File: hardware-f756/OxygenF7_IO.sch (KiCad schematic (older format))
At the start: 25 parts, among them J10 Micro_SD_Card_Det, J3 JST SH-4, J4 JST ZH-4, J5 Conn_03x08, J6 Conn_01x16, J7 Conn_01x04, J9 1.25mm, U3 MPU-6000, U4 BMP388, U5 W25Q128JVS

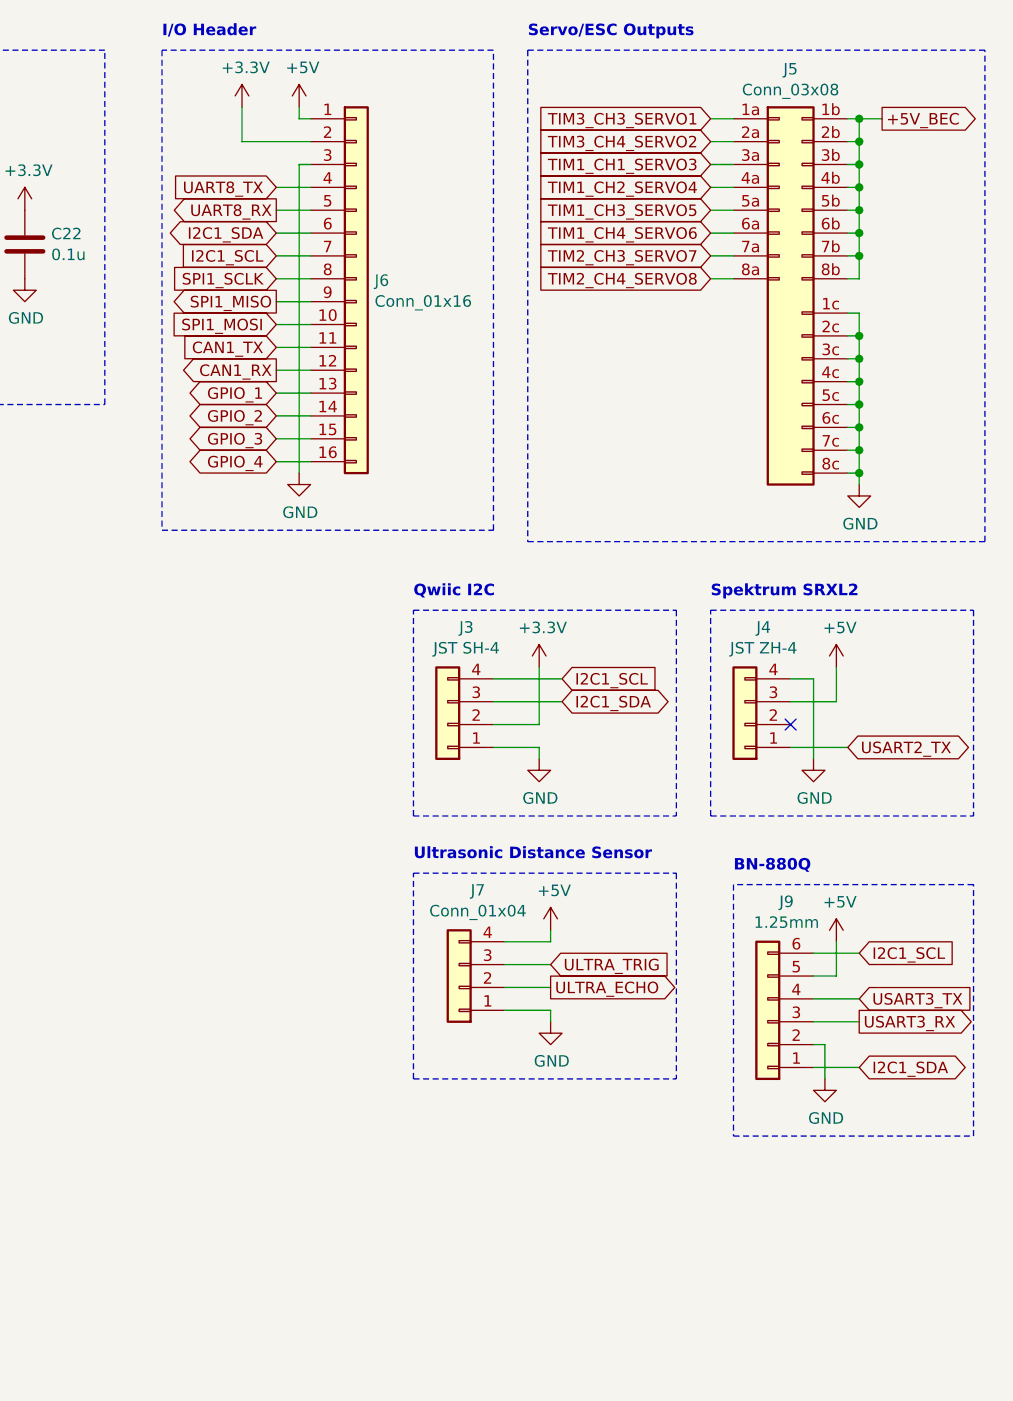
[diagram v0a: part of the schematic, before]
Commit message: New board layout
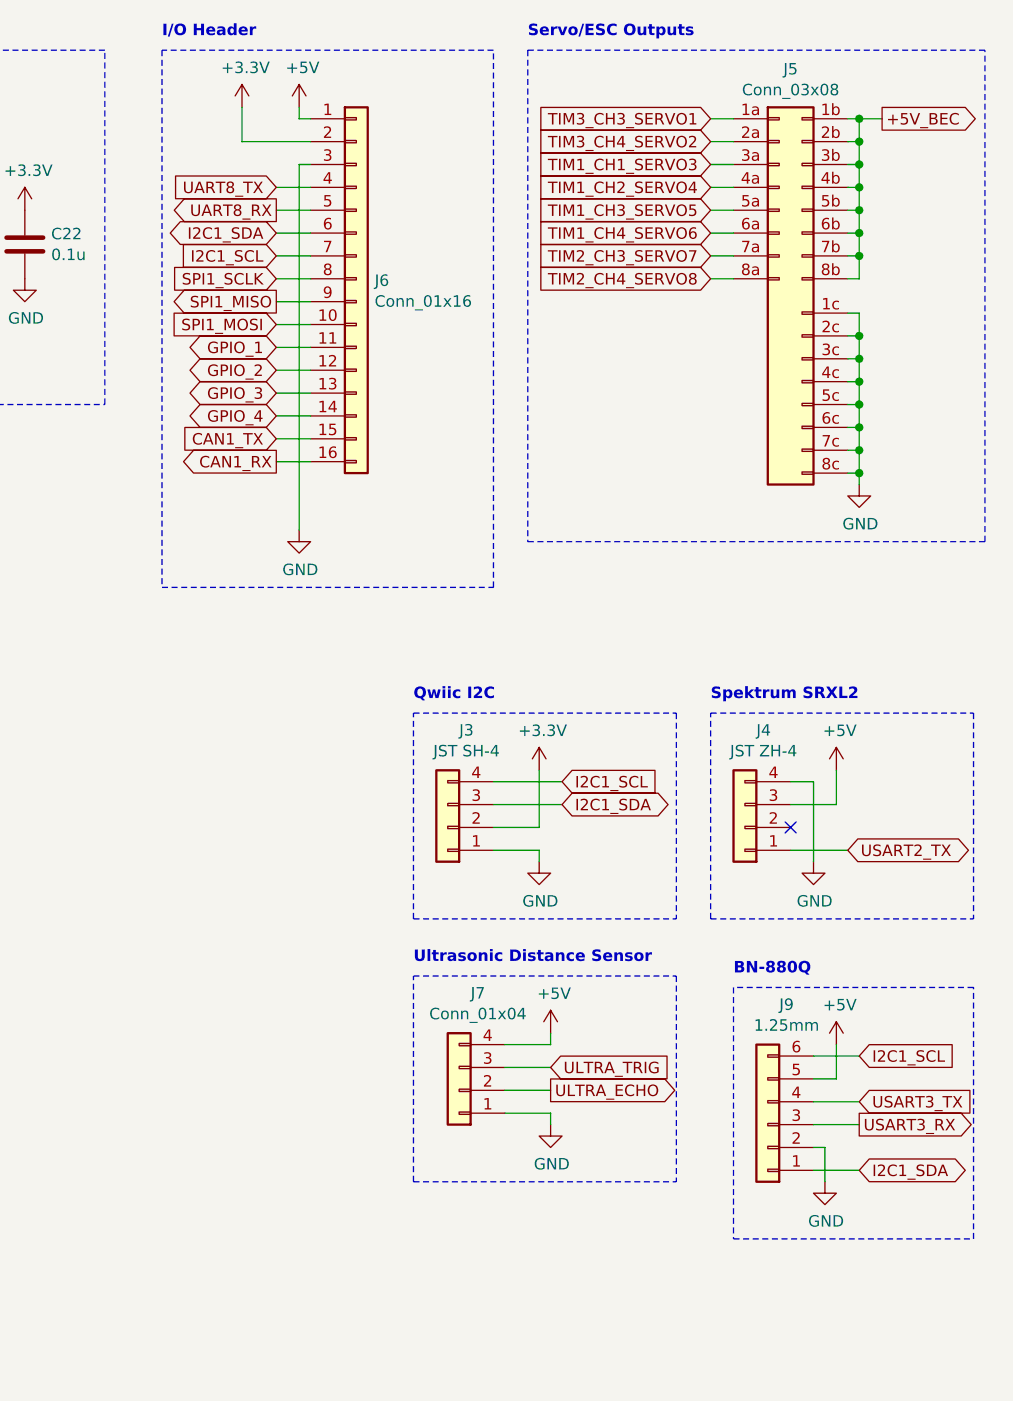
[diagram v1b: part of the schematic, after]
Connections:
- net CAN1_RX: now also J6.16 (Pin_16); no longer J6.12 (Pin_12)
- net CAN1_TX: now also J6.15 (Pin_15); no longer J6.11 (Pin_11)
- net GPIO_1: now also J6.11 (Pin_11); no longer J6.13 (Pin_13)
- net GPIO_2: now also J6.12 (Pin_12); no longer J6.14 (Pin_14)
- net GPIO_3: now also J6.13 (Pin_13); no longer J6.15 (Pin_15)
- net GPIO_4: now also J6.14 (Pin_14); no longer J6.16 (Pin_16)
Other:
- moved on the sheet: J3, J4, J7, J9
